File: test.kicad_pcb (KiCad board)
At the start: 2 copper layers, 44.4 x 26.5 mm, 2 parts

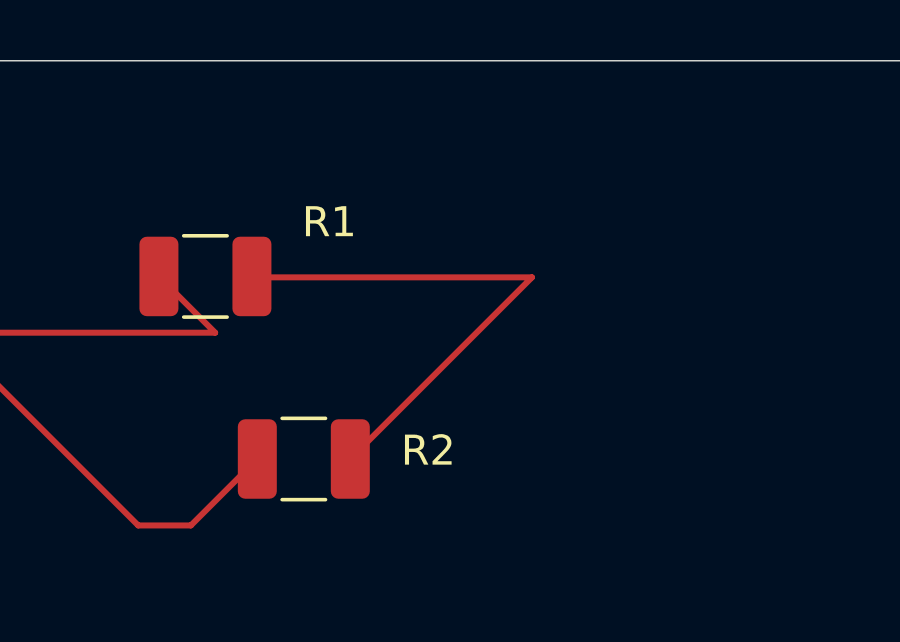
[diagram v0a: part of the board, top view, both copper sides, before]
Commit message: update pcb
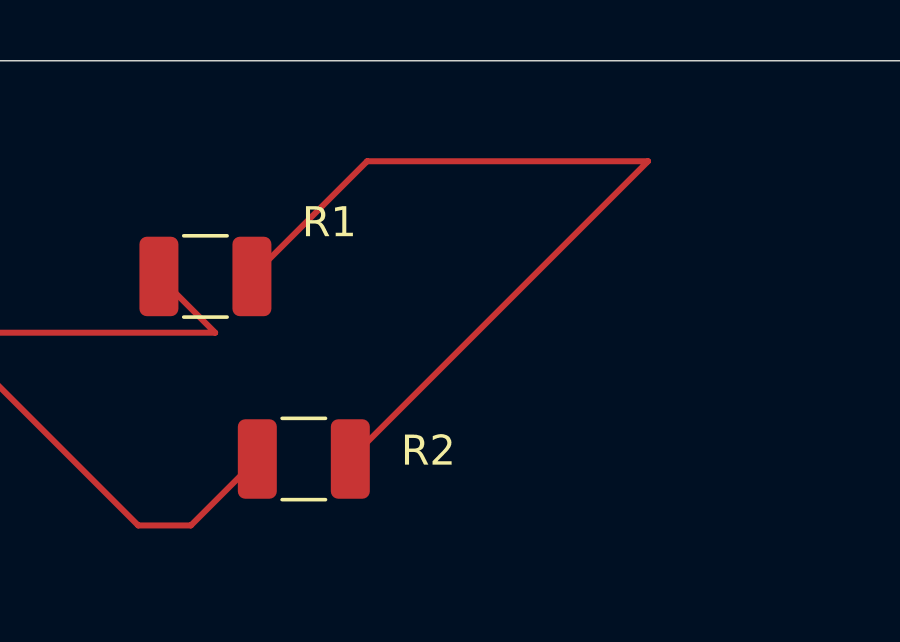
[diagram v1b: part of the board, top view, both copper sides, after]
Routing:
- net Net-(R1-Pad2): track 17.9 -> 28.8 mm
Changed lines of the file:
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@@
 	)
 	(segment
-		(start 151.085 80.51)
+		(start 141.75 80.48)
+		(end 145.59 76.64)
+		(width 0.2)
+		(layer "F.Cu")
+		(net 1)
+	)
+	(segment
+		(start 154.955 76.64)
 		(end 145.03 86.565)
 		(width 0.2)
@@
 	)
 	(segment
-		(start 141.78 80.51)
-		(end 151.085 80.51)
+		(start 145.59 76.64)
+		(end 154.955 76.64)
 		(width 0.2)
 		(layer "F.Cu")
-		(net 1)
-	)
-	(segment
-		(start 141.75 80.48)
-		(end 141.78 80.51)
-		(width 0.2)
-		(layer "F.Cu")

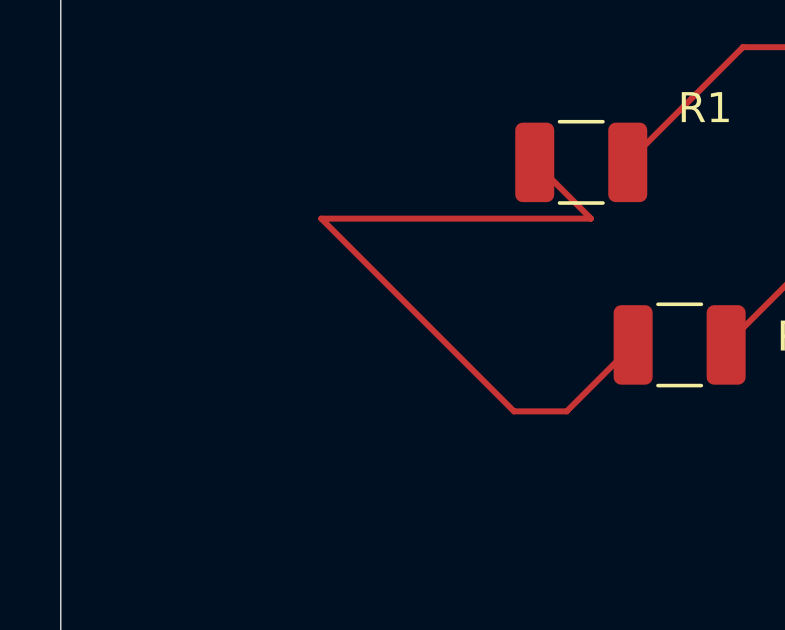
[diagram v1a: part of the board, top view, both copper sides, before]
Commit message: update pcb
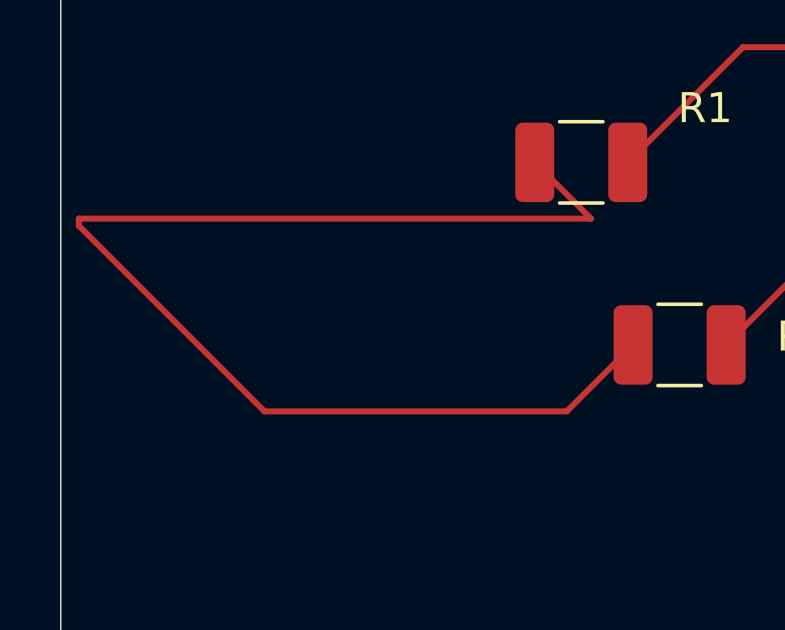
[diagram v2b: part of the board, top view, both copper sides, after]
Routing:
- net Net-(R1-Pad1): track 25.6 -> 41.9 mm
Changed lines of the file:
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@@
+	)
+	(segment
+		(start 129.64 88.78)
+		(end 139.715 88.78)
+		(width 0.2)
+		(layer "F.Cu")
+		(net 2)
 	)
 	(segment
@@
 	)
 	(segment
-		(start 140.525 82.355)
-		(end 131.535 82.355)
-		(width 0.2)
-		(layer "F.Cu")
-		(net 2)
-	)
-	(segment
-		(start 131.535 82.355)
-		(end 137.96 88.78)
-		(width 0.2)
-		(layer "F.Cu")
-		(net 2)
-	)
-	(segment
-		(start 137.96 88.78)
-		(end 139.715 88.78)
+		(start 123.451 82.355)
+		(end 123.451 82.591)
 		(width 0.2)
 		(layer "F.Cu")
@@
 		(width 0.2)
 		(layer "F.Cu")
+		(net 2)
+	)
+	(segment
+		(start 140.525 82.355)
+		(end 123.451 82.355)
+		(width 0.2)
+		(layer "F.Cu")
+		(net 2)
+	)
+	(segment
+		(start 123.451 82.591)
+		(end 129.64 88.78)
+		(width 0.2)
+		(layer "F.Cu")
